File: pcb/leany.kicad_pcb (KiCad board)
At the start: 2 copper layers, 89.4 x 69 mm, 73 parts, among them J1 ST7735S, J2 SWD, J3 USB C, J4 BATT, Q1 AO3401A, Q2 AO3400A, Q3 AO3401A, SW1 ZERO, SW2 HOLD, SW3 RESET, SW4 FLASH, SW5 POWER, U1 STM32F103C8Tx, U2 CH340C, U3 BMI270, U4 BQ25619, U5 AP2112K-3.3, Y1 8MHz

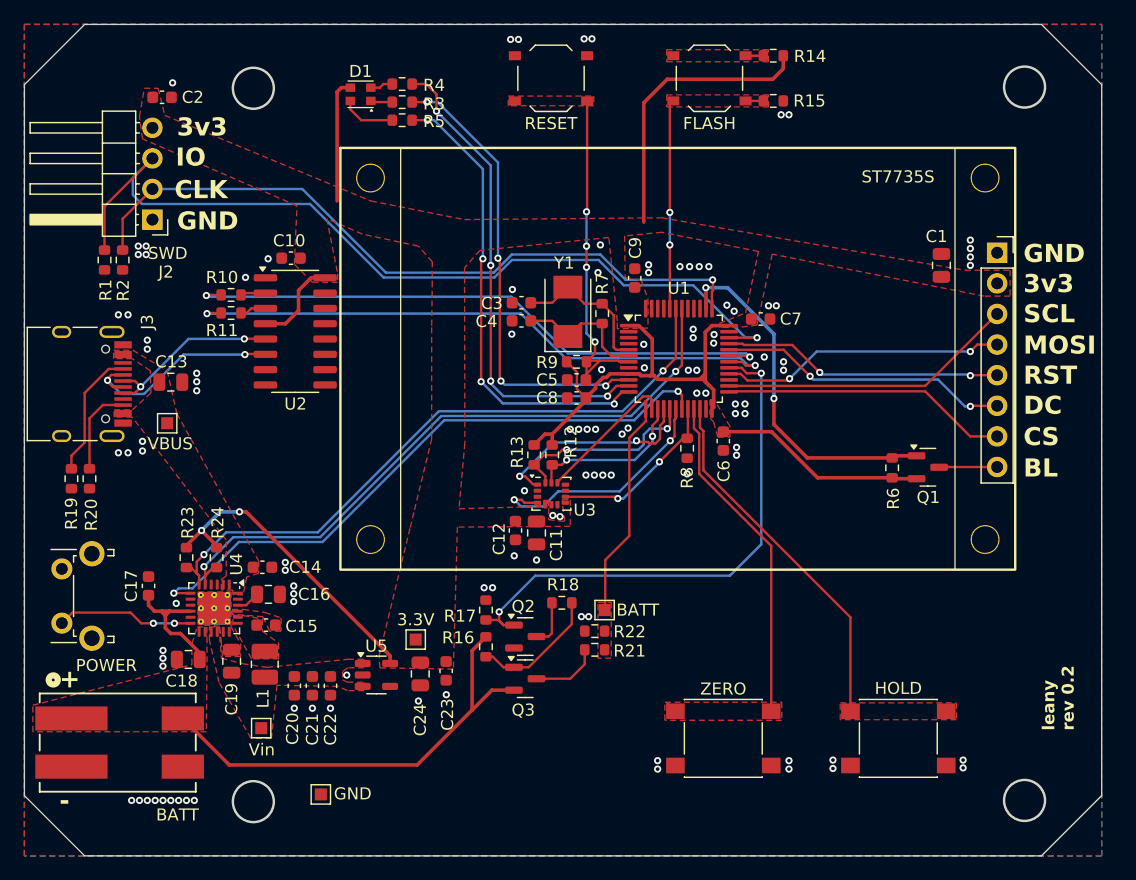
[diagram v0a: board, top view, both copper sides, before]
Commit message: feat: design PCB rev0.3 (#27)
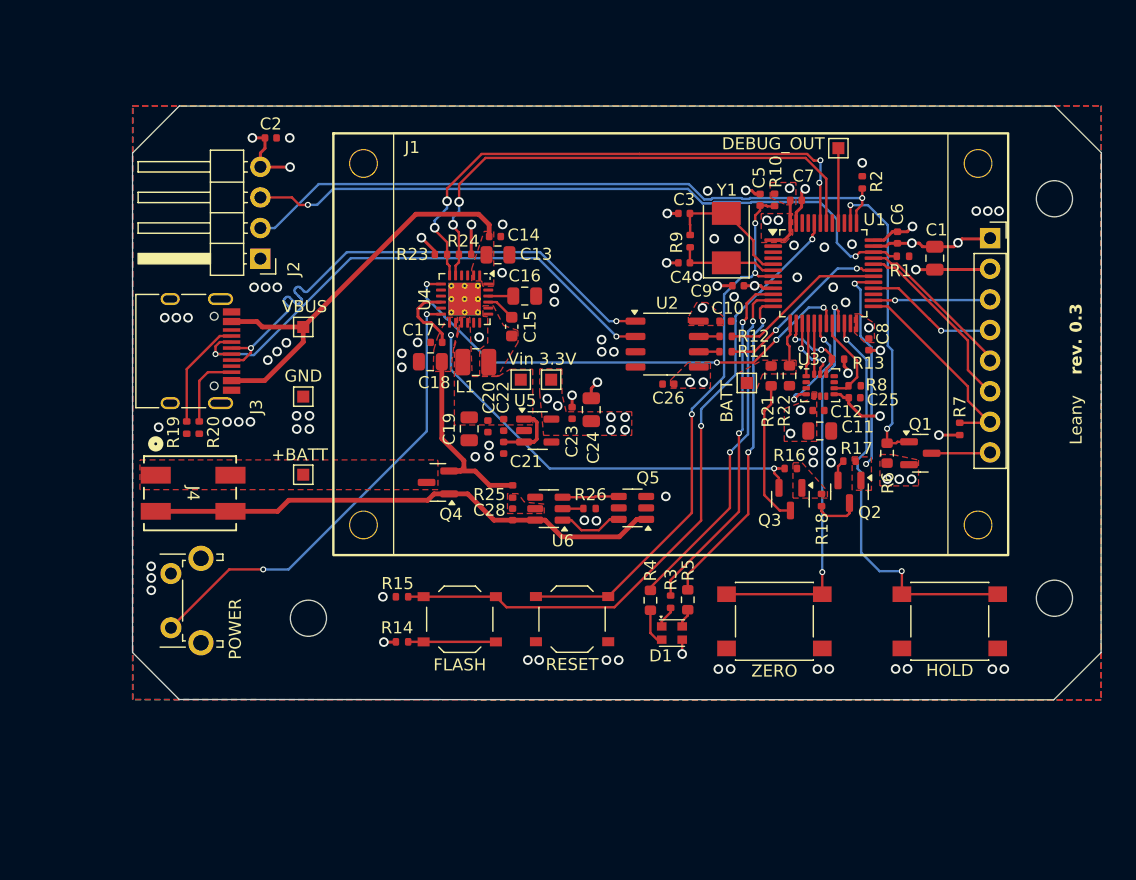
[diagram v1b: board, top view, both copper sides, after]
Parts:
- added C25: 100n, leany_footprints:C_0402_1005Metric, F.Cu at (164.9, 103.5)
- added C26: 100n, leany_footprints:C_0402_1005Metric, F.Cu at (149.4, 102.3)
- added C28: 100n, leany_footprints:C_0402_1005Metric, F.Cu at (136.5, 113.2)
- added Q4: AO3401A, Package_TO_SOT_SMD:SOT-23, F.Cu at (130.3, 110.5)
- added Q5: PT8810, Package_TO_SOT_SMD:SOT-23-6, F.Cu at (146.5, 112.6)
- added R25: 100R, leany_footprints:R_0402_1005Metric, F.Cu at (136.5, 111.3)
- added R26: 1k, leany_footprints:R_0402_1005Metric, F.Cu at (142.9, 112.7)
- added REF**: MountingHole_3mm, MountingHole:MountingHole_3mm, F.Cu at (119.6, 121.8)
- added REF**: MountingHole_3mm, MountingHole:MountingHole_3mm, F.Cu at (181.5, 87.0)
- added REF**: MountingHole_3mm, MountingHole:MountingHole_3mm, F.Cu at (181.5, 120.1)
- added TP6: Vin, leany_footprints:TestPoint_Pad_1.0x1.0mm, F.Cu at (137.2, 102.0)
- added TP7: 3.3V, leany_footprints:TestPoint_Pad_1.0x1.0mm, F.Cu at (139.7, 102.0)
- added U6: DW01A, Package_TO_SOT_SMD:SOT-23-6, F.Cu at (139.5, 112.7)
- C10, C12, C14, C17, C2, C20, C21, C22, C23, C3, C4, C5, C6, C7, C8, C9: footprint Capacitor_SMD:C_0603_1608Metric -> leany_footprints:C_0402_1005Metric
- J3: footprint Connector_USB:USB_C_Receptacle_HRO_TYPE-C-31-M-12 -> leany_footprints:USB_C_Receptacle_HRO_TYPE-C-31-M-12
- J4: footprint leany_footprints:wago_2060-452_998-404 -> leany_footprints:wago_2059-302_998-403
- R1, R11, R13, R14, R15, R16, R17, R18, R19, R2, R20, R23, R24, R3, R8: footprint Resistor_SMD:R_0603_1608Metric -> leany_footprints:R_0402_1005Metric
- R10: value 4k7 -> 10k; footprint Resistor_SMD:R_0603_1608Metric -> leany_footprints:R_0402_1005Metric
- R12: value 10k -> 4k7; footprint Resistor_SMD:R_0603_1608Metric -> leany_footprints:R_0402_1005Metric
- R7: value 1M -> 10k; footprint Resistor_SMD:R_0603_1608Metric -> leany_footprints:R_0402_1005Metric
- R9: value 10k -> 1M; footprint Resistor_SMD:R_0603_1608Metric -> leany_footprints:R_0402_1005Metric
- SW1: value ZERO -> SW_HIGH
- SW2: value HOLD -> SW_HIGH
- SW3: value RESET -> SW_LOW; footprint Button_Switch_SMD:SW_Push_1P1T_XKB_TS-1187A -> leany_footprints:SW_Push_1P1T_XKB_TS-1187A
- SW4: value FLASH -> SW_LOW; footprint Button_Switch_SMD:SW_Push_1P1T_XKB_TS-1187A -> leany_footprints:SW_Push_1P1T_XKB_TS-1187A
- TP1: value GND -> DEBUG_OUT
- TP2: value VBUS -> GND
- TP3: value BATT -> VBUS
- TP4: value Vin -> BATT
- TP5: value 3.3V -> +BATT
- U2: value CH340C -> CH340N; footprint Package_SO:SOIC-16_3.9x9.9mm_P1.27mm -> leany_footprints:SOP-8_3.9x4.9mm_P1.27mm
- U3: value BMI270 -> ICM-42688-P
- U5: footprint leany_footprints:TSOT-23-5 -> Package_TO_SOT_SMD:SOT-23-5
- moved TP1 68.7 mm to (163.6, 82.8)
- moved R1 66.3 mm to (168.9, 91.7), turned to 0 degrees
- moved R2 61.7 mm to (165.5, 85.6), turned to 90 degrees
- moved R14 57.6 mm to (127.3, 123.7), turned to 0 degrees
- moved D1 51.6 mm to (149.7, 123.0), turned to 180 degrees
- moved R15 51.4 mm to (127.3, 120.0), turned to 180 degrees
- moved SW4 49.4 mm to (132.1, 121.9), turned to 180 degrees
- moved TP4 49.4 mm to (155.9, 102.3), turned to 180 degrees
- moved R4 47.5 mm to (147.9, 120.3), turned to 90 degrees
- moved R3 47.1 mm to (149.6, 120.4), turned to 90 degrees
- moved R5 46.3 mm to (151.1, 120.2), turned to 90 degrees
- moved R10 45.8 mm to (158.2, 87.1), turned to -90 degrees
- moved SW3 44.9 mm to (141.4, 121.9), turned to 180 degrees
- moved R11 41.2 mm to (154.2, 99.7), turned to 180 degrees
- moved C10 36.4 mm to (154.2, 97.1), turned to 0 degrees
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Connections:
- net /BMI270_INT1 renamed /IMU_INT1
- net /BMI270_INT2 renamed /IMU_INT2
- net /BMI270_SDO renamed /IMU_MISO
- J4 pad 1: +BATT -> Net-(J4-1_1)
- J4 pad 2: +BATT -> Net-(J4-1_1)
- J4 pad 3: GND -> GNDREF
- J4 pad 4: GND -> GNDREF
- R10 pad 1: /FTDI_RX -> +3V3
- R10 pad 2: Net-(U2-TXD) -> Net-(U1-NRST)
- R11 pad 1: /FTDI_TX -> /FTDI_RX
- R11 pad 2: Net-(U2-RXD) -> Net-(U2-TXD)
- R12 pad 1: +3V3 -> /FTDI_TX
- R12 pad 2: /BMI270_SCL -> Net-(U2-RXD)
- R13 pad 2: /BMI270_SDA -> /IMU_CS
- R7 pad 1: Net-(U1-PD0) -> +3V3
- R7 pad 2: Net-(U1-PD1) -> /ST7735S_CS
- R9 pad 1: +3V3 -> Net-(U1-PD0)
- R9 pad 2: Net-(U1-NRST) -> Net-(U1-PD1)
- TP1 pad 1: GND -> /DEBUG_OUT
- TP2 pad 1: Net-(U4-PSEL) -> GND
- TP3 pad 1: BATT_VOLT -> Net-(U4-PSEL)
- TP4 pad 1: SYS -> BATT_VOLT
- TP5 pad 1: +3V3 -> Net-(J4-1_1)
- U1 pad 14: /BMI270_CS -> /IMU_CS
- U1 pad 15: /BMI270_SCL -> /IMU_SCK
- U1 pad 17: /BMI270_SDA -> /IMU_MOSI
- U1 pad 40: unconnected-(U1-PB4-Pad40) -> /DEBUG_OUT
- U2 pad 1: GND -> USB_D+
- U2 pad 2: Net-(U2-TXD) -> USB_D-
- U2 pad 3: Net-(U2-RXD) -> GND
- U2 pad 4: +3V3 -> unconnected-(U2-~{RTS}-Pad4)
- U2 pad 5: USB_D+ -> +3V3
- U2 pad 6: USB_D- -> Net-(U2-TXD)
- U2 pad 7: unconnected-(U2-NC-Pad7) -> Net-(U2-RXD)
- U2 pad 8: unconnected-(U2-NC-Pad8) -> +3V3
- U3 pad 12: /BMI270_CS -> /IMU_CS
- U3 pad 13: /BMI270_SCL -> /IMU_SCK
- U3 pad 14: /BMI270_SDA -> /IMU_MOSI
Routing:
- net +3V3: track 122.6 -> 37.4 mm, vias 2 -> 30
- net GNDREF: track 0.00 -> 43.4 mm
- net /BOOT0: track 18.8 -> 56.3 mm
- net /FTDI_TX: track 50.7 -> 13.8 mm, vias 2 -> 0
- net /FTDI_RX: track 50.3 -> 14.7 mm
- net Net-(U4-PSEL): track 0.00 -> 35.3 mm
- net USB_D+: track 15.4 -> 44.7 mm
- net BATT_EN: track 44.9 -> 17.3 mm
- net Net-(U4-~{QON}): track 11.4 -> 38.9 mm
- net USB_D-: track 18.0 -> 44.4 mm
- net GND: track 0.00 -> 23.1 mm, vias 114 -> 80
- net Net-(U1-NRST): track 29.4 -> 47.0 mm, vias 4 -> 3
- net /BMI270_SDA: track 16.4 -> 0.00 mm, vias 2 -> 0
- net /DEBUG_SWDIO: track 73.2 -> 57.5 mm, vias 1 -> 2
- net /ST7735S_SCL: track 24.7 -> 9.74 mm, vias 0 -> 1
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- added copper zone on In2.Cu, net +3V3
- added copper zone on F.Cu, net BATT_EN
- added copper zone on In1.Cu, net GND
- added copper zone on F.Cu, net Net-(J4-1_1)
- added copper zone on F.Cu, net Net-(Q3-G)
- added copper zone on F.Cu, net Net-(U6-VCC)
- removed copper zone on F.Cu, net /BOOT0
- removed copper zone on F.Cu, net Net-(R14-Pad2)
- removed copper zone on F.Cu, net Net-(U1-NRST)
- removed copper zone on F.Cu, net Net-(U1-PB10)
- removed copper zone on F.Cu, net Net-(U1-PB11)
- removed copper zone on F.Cu, net Net-(U4-BTST)
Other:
- board size 89.4 x 69 mm -> 80.4 x 49.3 mm
- copper layers 2 -> 4
- board text added: "Leany"
- board text added: "rev. 0.3"
- board text removed: "+"
- board text removed: "-"
- board text removed: "3v3"
- board text removed: "BL"
- board text removed: "CLK"
- board text removed: "CS"
- board text removed: "DC"
- board text removed: "GND"
- board text removed: "IO"
- board text removed: "MOSI"
- board text removed: "RST"
- board text removed: "SCL"
- board text removed: "leany rev 0.2"
